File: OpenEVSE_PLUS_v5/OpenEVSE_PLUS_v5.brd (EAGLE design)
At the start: 65 x 44.9 mm, 72 parts, among them IC1 HCPL-2731, IC2 MEGA8-AI, IC3 LMV358, IC4 LMV358, IC5 AQH1213, Q1 16000, Q2 2222A, Q3 2222A

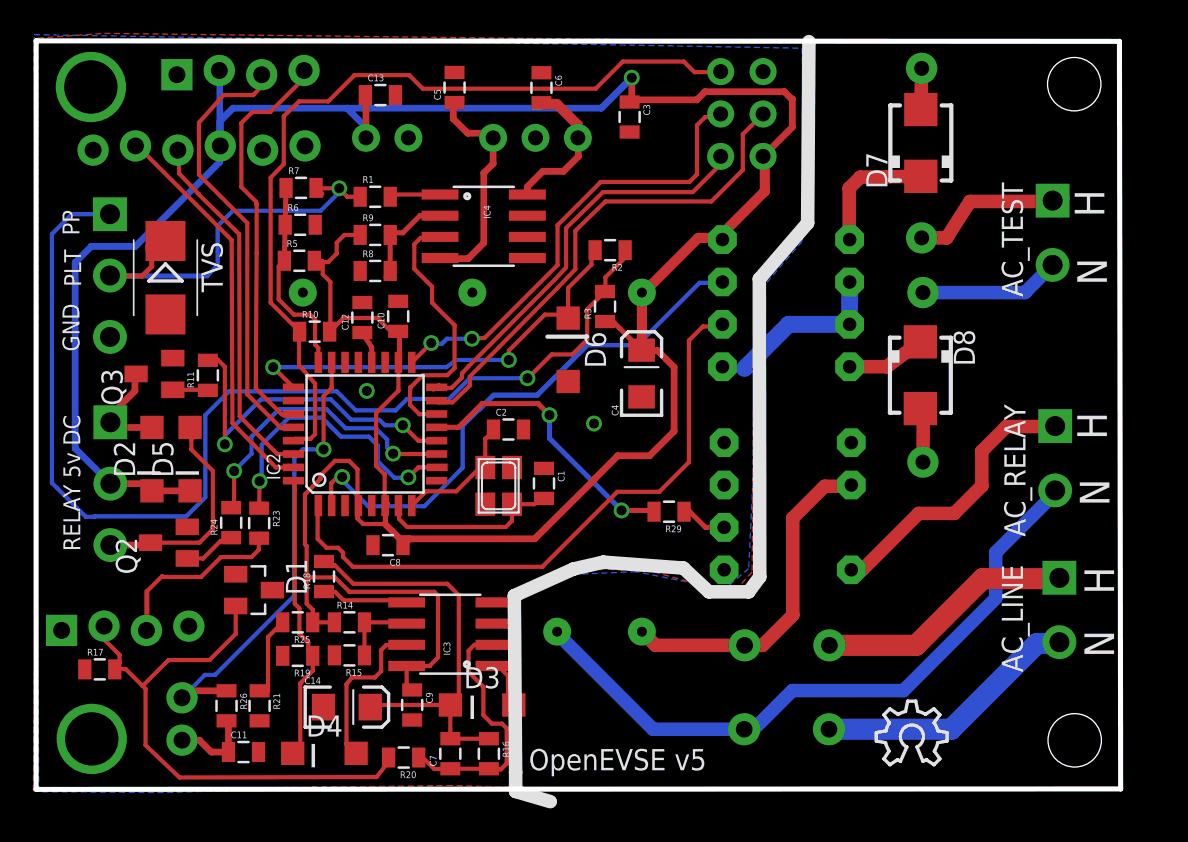
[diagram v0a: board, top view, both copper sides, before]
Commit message: v5
V5 files added
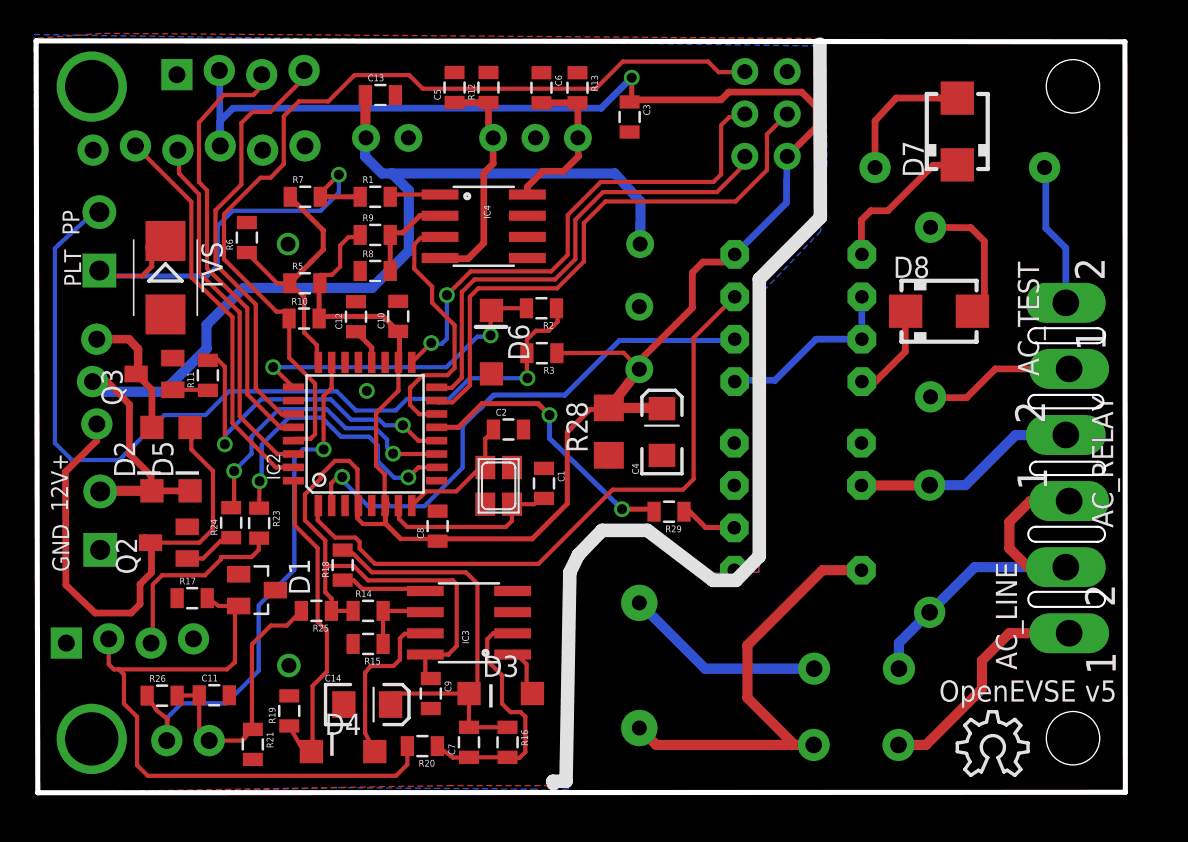
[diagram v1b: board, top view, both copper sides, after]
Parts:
- removed AC_LINE, AC_RELAY, AC_TEST: TE 1776275-2, SparkFun:SCREWTERMINAL-3.5MM-2_LOCK
- removed A_CT: (no value), SparkFun:1X02
- removed G_CT: G_CT, SparkFun:1X04_LOCK
- removed RELAY: (no value), SparkFun:SCREWTERMINAL-3.5MM-3_LOCK.007S
- added 12VDC: (no value), SparkFun-Connectors:SCREWTERMINAL-3.5MM-2
- added AC: JST-VH-6, OpenEVSE:JST-VH-6
- added AMP_CT: AMP_CT, OpenEVSE:MOLEX_2
- added DC_RELAY: DC_RELAY, OpenEVSE:MOLEX_3
- added GFCI_CT: GFCI_CT, OpenEVSE:GFCI_4
- added R12, R13: 2.4k, SparkFun:0805
- added R28: 180, rcl:R1206
- added U$1: MOV, OpenEVSE:MOV
- added U$3, U$4: HOLE, OpenEVSE:HOLE
- D1: value BAS40-06 -> AZ23C5V6-7-F
- DCDC: value D107E -> MD112D-12E
- IC2: value MEGA8-AI -> ATMEGA328P-AU
- IC3: value LMV358 -> LM358
- IC4: value LMV358 -> LF353
- PILOT: value Pilot -> (none); device SparkFun:SCREWTERMINAL-3.5MM-3_LOCK.007S -> SparkFun-Connectors:SCREWTERMINAL-3.5MM-2
- PS1: value AAF-05 -> MPM-04E-1205; device Qxd:AAF -> Qxd:MPM-04E-1205
- R1: value 650 -> 620
- R17: value GND -> 412
- R22: value 200k -> 200K
- R26: value 28 -> 22
- TVS: value P6SMB16A -> P6SMB16CA
- moved PS1 32.4 mm to (39.0, 0.10), turned to 0 degrees
- moved F2 7.26 mm to (44.8, 0.84)
- moved R17 6.99 mm to (9.17, 11.6)
- moved F1 5.55 mm to (44.8, 5.41)
- moved R2 5.39 mm to (30.1, 29.0)
- moved LOGO1 4.89 mm to (55.0, 1.02)
- moved R3 4.70 mm to (30.1, 26.3), turned to 180 degrees
- moved LOGO2 4.66 mm to (59.0, 0.94)
- moved D6 4.62 mm to (27.1, 27.0)
- moved D8 3.99 mm to (53.9, 28.8), turned to 0 degrees
- moved R22 3.94 mm to (53.4, 28.8), turned to 90 degrees
- moved R26 3.91 mm to (7.37, 5.79), turned to 0 degrees
- moved C11 3.83 mm to (10.5, 5.82)
- moved C4 3.71 mm to (37.3, 21.6)
- moved R19 3.34 mm to (15.0, 4.88), turned to 90 degrees
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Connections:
- removed net N$12 (its old number): AC_LINE.1, F2.OUT
- removed net N$13 (its old number): AC_LINE.2, F1.OUT
- removed net N$17 (its old number): AC_TEST.1, R4.P$1
- removed net N$29: AC_TEST.2, R22.P$1
- new net +12V: 12VDC.2, C13.1, D2.C, D5.C, DCDC.VIN+, DC_RELAY.2, PS1.12V
- new net ACIN1: AC.P$1, F2.OUT
- new net ACIN2: AC.P$2, AC.P$3, F1.OUT, U$1.P$1
- new net ACTEST1: AC.P$6, R4.P$1
- new net ACTEST2: AC.P$5, R22.P$1
- net +5V: now also PS1.5V, R28.2; no longer C13.1, D2.C, D5.C, DCDC.VIN+, PS1.P$5, RELAY.2
- net -12V: now also R12.1
- net 12V: now also R13.2
- net ACRELAY: now also AC.P$4, IC5.6, U$1.P$2; no longer AC_RELAY.1, IC5.8
- net AC_TEST: now also IC1.7; no longer IC1.6
- net AC_TEST_2: now also IC1.6; no longer IC1.7
- net AMP_READ: now also AMP_CT.2; no longer A_CT.1
- net FUSEL: now also IC5.8, PS1.ACL; no longer IC5.6, PS1.P$1
- net FUSEN: now also PS1.ACN; no longer AC_RELAY.2, PS1.P$2
- net GND: now also 12VDC.1, GFCI_CT.1, GFCI_CT.4, PS1.GND, R12.2, R13.1, R28.1, U$3.P$1, U$4.P$1; no longer G_CT.1, G_CT.4, PILOT.3, PS1.P$4
- net N$1: now also DC_RELAY.3; no longer RELAY.1
- net N$20: now also GFCI_CT.2; no longer G_CT.2
- net N$22: now also GFCI_CT.3; no longer G_CT.3
- net N$6: now also DC_RELAY.1; no longer RELAY.3
- net N$7: now also AMP_CT.1; no longer A_CT.2
- net PILOT: now also PILOT.1; no longer PILOT.2
- net PP: now also PILOT.2; no longer PILOT.1
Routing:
- net +12V: track 0.00 -> 67.2 mm
- net +5V: track 193.1 -> 158.4 mm
- net FUSEN: track 39.9 -> 12.1 mm
- net ACIN2: track 0.00 -> 23.0 mm
- net N$6: track 13.5 -> 31.4 mm
- net N$13 (its old number): track 16.0 -> 0.00 mm
- net N$12 (its old number): track 15.5 -> 0.00 mm
- net ACIN1: track 0.00 -> 14.0 mm
- net PP: track 66.4 -> 53.1 mm
- net N$17 (its old number): track 10.4 -> 0.00 mm
- net ACTEST2: track 0.00 -> 9.04 mm
- net ACTEST1: track 0.00 -> 8.63 mm
- net N$29: track 8.46 -> 0.00 mm
- net FUSEL: track 20.3 -> 26.7 mm
- net PP_READ: track 25.9 -> 19.6 mm
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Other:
- board size 65 x 44.9 mm -> 65.3 x 45.1 mm
- board text added: "12V DC Relay"
- board text added: "12V+"
- board text removed: "H"
- board text removed: "IC1"
- board text removed: "IC6"
- board text removed: "N"
- board text removed: "RELAY 5v DC"
